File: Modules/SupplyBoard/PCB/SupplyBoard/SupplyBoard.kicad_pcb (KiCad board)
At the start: 2 copper layers, 60 x 80 mm, 83 parts, among them J1 CI_BATT, J2 SW-DP, J3 CIO_MAIN_CONNECTOR, Q1 AGP30P35AP, Q2 IRLM2502, SW1 RESET, SW2 SW_SPDT_312, U1 STM32L031G6Ux, U2 TPS63070, U6 TMP20AIDCK

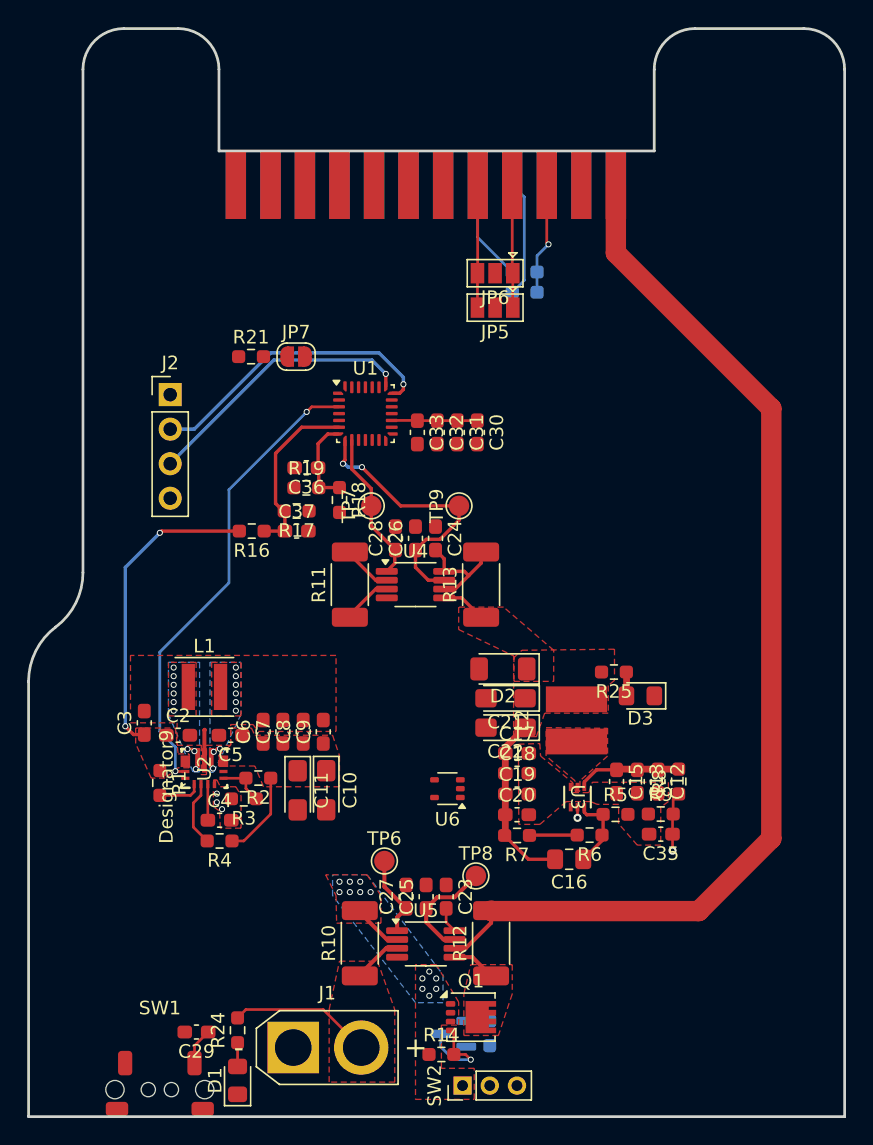
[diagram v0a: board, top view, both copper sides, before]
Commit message: Finished Supply board
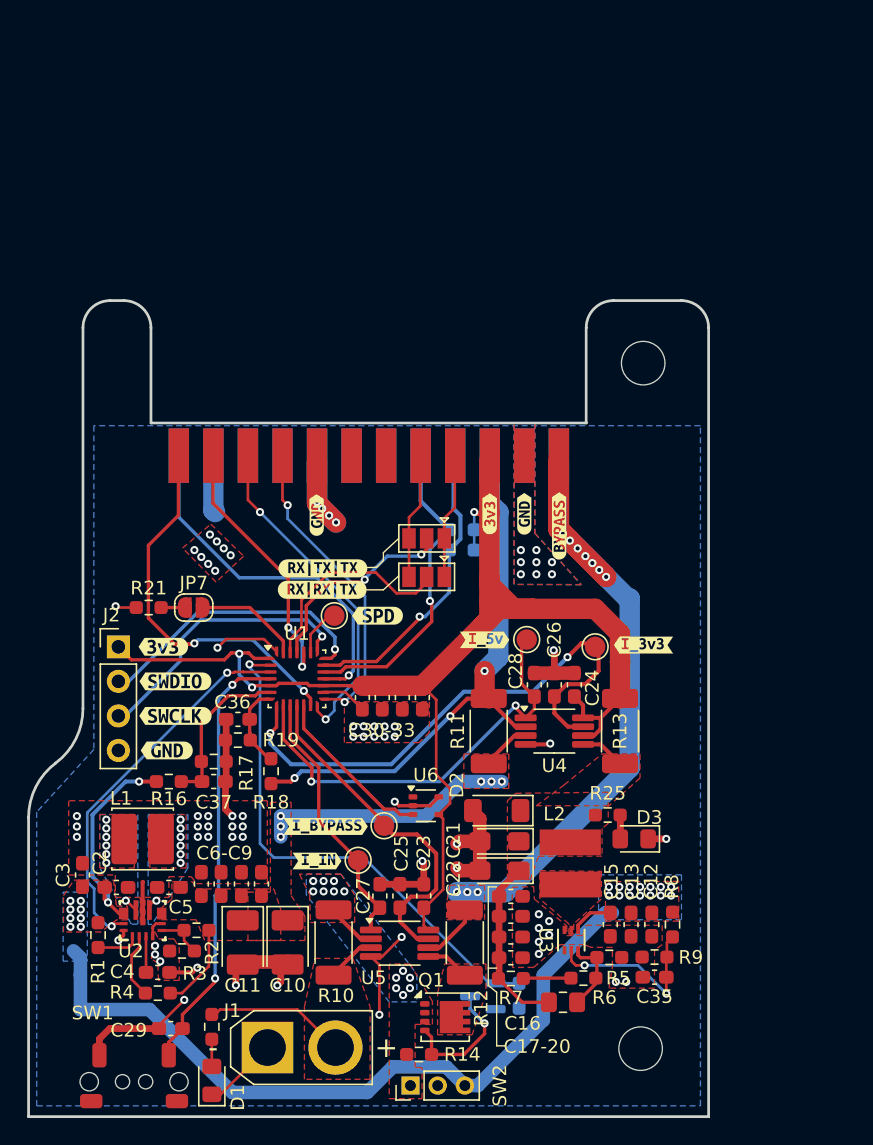
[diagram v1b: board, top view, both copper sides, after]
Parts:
- added G***: LOGO, IcaroFootprints:LogoGluon_12mm, B.Cu at (158.8, 92.7)
- added REF**: MountingHole_3.2mm_M3_DIN965, MountingHole:MountingHole_3.2mm_M3_DIN965, F.Cu at (197.6, 46.2)
- added REF**: MountingHole_3.2mm_M3_DIN965, MountingHole:MountingHole_3.2mm_M3_DIN965, F.Cu at (197.4, 96.6)
- added REF**: KiCad-Logo2_5mm_SilkScreen, Symbol:KiCad-Logo2_5mm_SilkScreen, B.Cu at (197.5, 57.8)
- added TP1: STM_SPEED, TestPoint:TestPoint_Pad_D1.5mm, F.Cu at (174.9, 64.8)
- added kibuzzard-67BD8B4D: G***, kibuzzard-67BD8B4D, F.Cu at (174.0, 61.3)
- added kibuzzard-67BD8B63: G***, kibuzzard-67BD8B63, F.Cu at (174.0, 62.9)
- added kibuzzard-67BD8B96: G***, kibuzzard-67BD8B96, F.Cu at (186.3, 57.3)
- added kibuzzard-67BD8B9D: G***, kibuzzard-67BD8B9D, F.Cu at (191.4, 58.2)
- added kibuzzard-67BD8B9D: G***, kibuzzard-67BD8B9D, B.Cu at (191.4, 60.0)
- added kibuzzard-67BD8BAB: G***, kibuzzard-67BD8BAB, F.Cu at (188.8, 57.3)
- added kibuzzard-67BD8BAB: G***, kibuzzard-67BD8BAB, F.Cu at (173.6, 57.4)
- added kibuzzard-67BD8C21: G***, kibuzzard-67BD8C21, B.Cu at (186.3, 57.0)
- added kibuzzard-67BD8C4F: G***, kibuzzard-67BD8C4F, B.Cu at (173.6, 57.3)
- added kibuzzard-67BD8C4F: G***, kibuzzard-67BD8C4F, B.Cu at (188.8, 57.3)
- added kibuzzard-67BD8C4F: G***, kibuzzard-67BD8C4F, B.Cu at (166.0, 57.2)
- added kibuzzard-67BD8EAE: G***, kibuzzard-67BD8EAE, F.Cu at (173.6, 82.8)
- added kibuzzard-67BD8EBE: G***, kibuzzard-67BD8EBE, F.Cu at (174.2, 80.3)
- added kibuzzard-67BD8ECC: G***, kibuzzard-67BD8ECC, F.Cu at (185.9, 66.5)
- added kibuzzard-67BD8EE5: G***, kibuzzard-67BD8EE5, F.Cu at (197.6, 66.9)
- added kibuzzard-67BD90D0: G***, kibuzzard-67BD90D0, F.Cu at (163.2, 69.6)
- added kibuzzard-67BD90D4: G***, kibuzzard-67BD90D4, F.Cu at (163.2, 72.1)
- added kibuzzard-67BD90DE: G***, kibuzzard-67BD90DE, F.Cu at (162.3, 67.1)
- added kibuzzard-67BD90E3: G***, kibuzzard-67BD90E3, F.Cu at (162.6, 74.7)
- added kibuzzard-67BD93F4: G***, kibuzzard-67BD93F4, B.Cu at (185.1, 63.7)
- added kibuzzard-67BDA321: G***, kibuzzard-67BDA321, F.Cu at (178.1, 64.8)
- C10, C11: footprint Capacitor_Tantalum_SMD:CP_EIA-3216-18_Kemet-A_Pad1.58x1.35mm_HandSolder -> Capacitor_Tantalum_SMD:CP_EIA-3528-21_Kemet-B_Pad1.50x2.35mm_HandSolder
- L1: footprint Inductor_SMD:L_Coilcraft_XxL4040 -> Inductor_SMD:L_Cenker_CKCS4030
- moved J3 20.8 mm to (177.4, 53.5)
- moved R18 20.6 mm to (170.2, 76.2)
- moved JP5 20.4 mm to (181.7, 61.9)
- moved JP6 20.1 mm to (181.7, 59.1)
- moved U1 20.1 mm to (172.1, 69.4)
- moved JP7 19.9 mm to (164.5, 64.2)
- moved R21 19.9 mm to (161.2, 64.2)
- moved C30 19.9 mm to (181.4, 70.8)
- moved C31 19.9 mm to (179.9, 70.8)
- moved C32 19.9 mm to (178.4, 70.8)
- moved C33 19.9 mm to (176.9, 70.8)
- moved R22 19.5 mm to (184.3, 59.9)
- moved R23 19.5 mm to (184.3, 58.4)
- moved C37 19.4 mm to (166.0, 77.0)
- moved R16 19.4 mm to (162.7, 77.0)
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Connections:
- U1 pad 14: /SPI.MOSI -> /SPI.MISO
- U1 pad 15: /SPI.MISO -> /SPI.MOSI
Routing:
- net GND: track 2.26 -> 91.5 mm, vias 3 -> 72
- net +3.3V: track 24.6 -> 101.1 mm, vias 1 -> 3
- net /Controlador/BATT_INPUT: track 30.6 -> 73.9 mm, vias 2 -> 24
- net +5V: track 3.67 -> 40.8 mm, vias 0 -> 3
- net /BYPASS_EN: track 1.73 -> 38.4 mm, vias 0 -> 1
- net /Controlador/~{RESET}: track 2.70 -> 32.2 mm, vias 0 -> 2
- net /SPI.CS0: track 0.00 -> 29.2 mm, vias 0 -> 2
- net /SPI.CS1: track 0.00 -> 26.8 mm, vias 0 -> 1
- net /SPI.MISO: track 0.00 -> 25.0 mm, vias 0 -> 2
- net /SPI.MOSI: track 0.00 -> 22.9 mm, vias 0 -> 2
- net /I_{3v3}_SENSE: track 20.5 -> 40.9 mm
- net /I_{5v}_SENSE: track 11.3 -> 31.6 mm, vias 0 -> 2
- net /SPI.SCK: track 0.00 -> 19.2 mm, vias 0 -> 2
- net /LIPO_TO_5V/5V_OUT: track 9.98 -> 28.9 mm, vias 0 -> 6
- net /I_{BYPASS}_SENSE: track 8.27 -> 26.7 mm
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- added copper zone on F.Cu, net /BATT_BYPASS
- added copper zone on B.Cu, net /Controlador/BATT_INPUT
- added copper zone on B.Cu, net GND
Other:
- board size 60 x 80 mm -> 50 x 60 mm
- board text added: "C17-20"
- board text added: "C30-33"
- board text added: "C6-C9"
- board text added: "Gracias a todos:"
- board text added: "Proyecto Ícaro SupplyBoard V1.0 by: @labgluon"
- board text added: "gordon_clark movich4 adiiran pulwef kerneltron victor_gomezzz dhontecillas pintzio2 bark12 alnaumiwebs"
- board text added: "laboratoriocautin qvision_dev tuboniatofugaz t3l3mac0 rafaromevi hec100h diegomallo jsochoa crovodovod joseju_ch"
- board text added: "spuertes araba_st zurano_ carlosbetdev gorn6_ david_wiki sergivv txusev enlopa blacai"
